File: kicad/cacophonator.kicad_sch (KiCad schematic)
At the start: 53 parts, among them J1 Jack-DC, J2 AUDIO OUTPUT, SW1 POWER, SW2 CHARGE, U1 40106

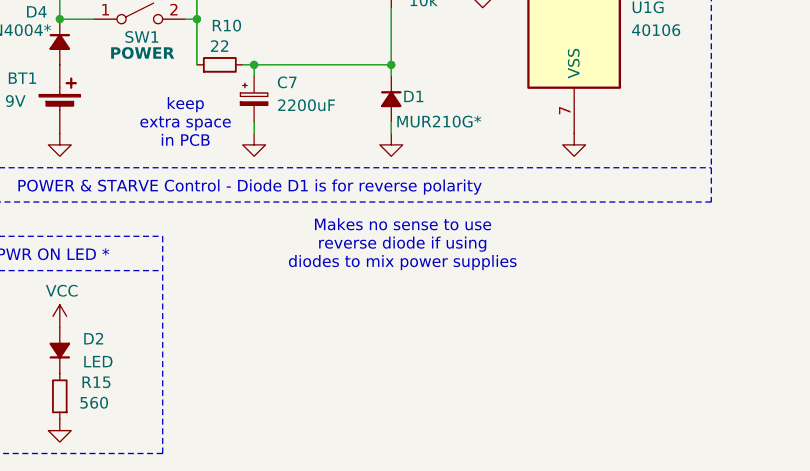
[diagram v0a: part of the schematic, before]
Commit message: Minor updates
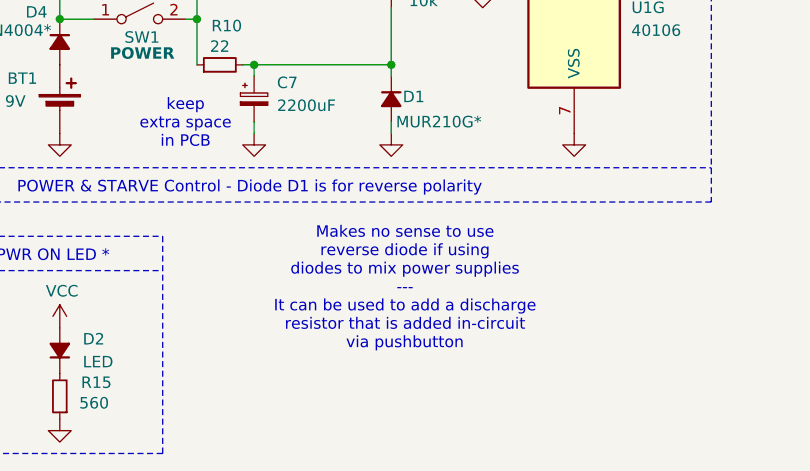
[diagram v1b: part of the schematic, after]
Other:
- note added: "Makes no sense to use reverse diode if using diodes to mix power supplies --- It can be used to add a discharge resistor that is added in-circuit via pushbutton"
- note removed: "Makes no sense to use reverse diode if using diodes to mix power supplies"
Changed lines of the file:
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@@
 		)
 	)
-	(text "Makes no sense to use\nreverse diode if using \ndiodes to mix power supplies"
+	(text "Makes no sense to use\nreverse diode if using \ndiodes to mix power supplies\n---\nIt can be used to add a discharge\nresistor that is added in-circuit\nvia pushbutton"
 		(exclude_from_sim no)
-		(at 107.95 161.036 0)
+		(at 108.204 165.862 0)
 		(effects
 			(font
